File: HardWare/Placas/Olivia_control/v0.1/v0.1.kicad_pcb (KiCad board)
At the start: 2 copper layers, 100 x 100 mm, 47 parts, among them J1 PROG, J10 Motor_B, J11 I2C, J12 DAC, J13 UART2, J15 TRIAC_220VAC, J17 In12V, J2 Input1, J3 Input2, J4 Input3, J5 Input4, J6 LED, J7 Reset, J8 SPI, J9 Motor_A, Q1 BTA16-800B, Q2 BTA16-800B, U1 ESP32-WROOM-32D, U2 MOC3041M, U3 MOC3041M, U4 4N25, U5 AMS1117-3.3, U6 HW-613

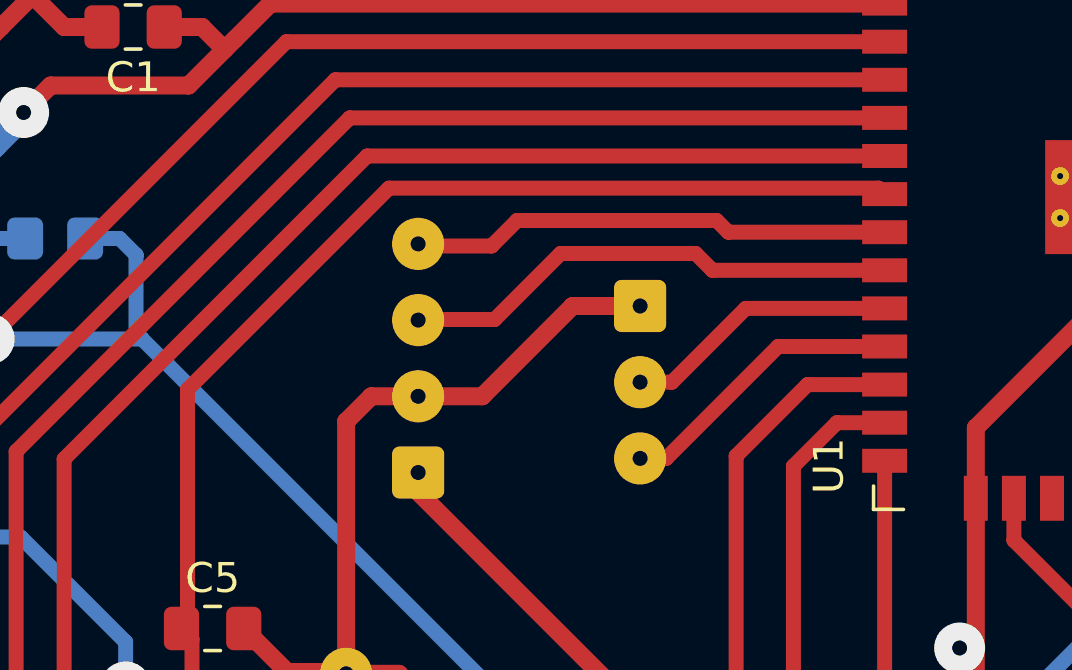
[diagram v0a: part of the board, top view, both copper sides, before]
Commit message: minor fix
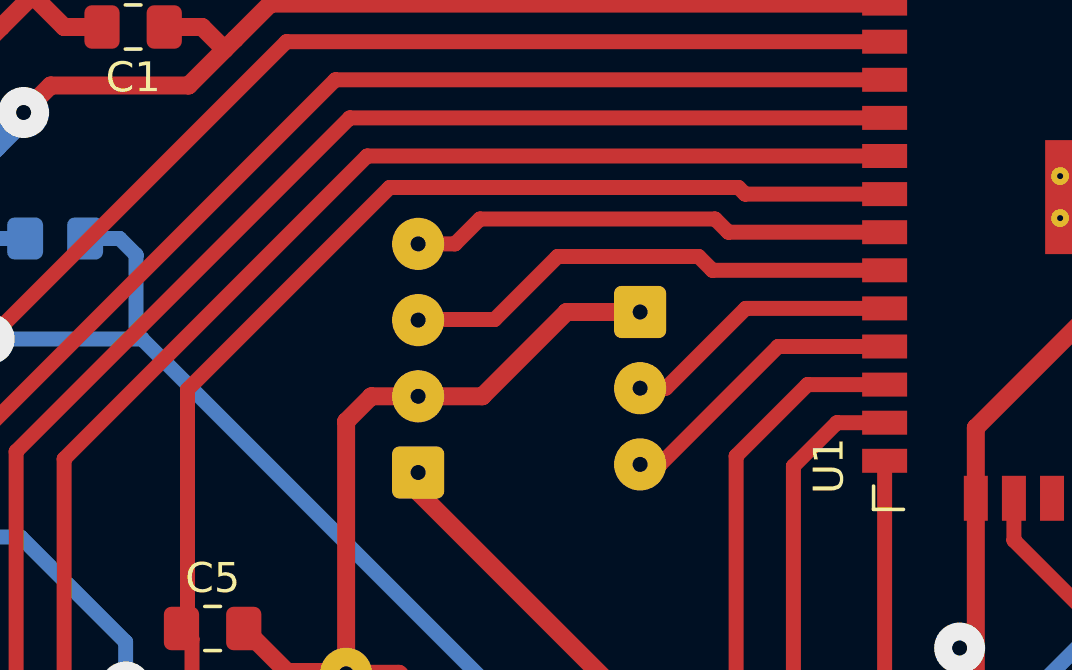
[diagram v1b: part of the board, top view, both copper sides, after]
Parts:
- moved J12 0.20 mm to (129.8, 58.1)
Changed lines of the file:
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@@
 		(allow_soldermask_bridges_in_footprints no)
 		(pcbplotparams
-			(layerselection 0x0000000_fffffffe)
+			(layerselection 0x0000000_7fffffff)
 			(plot_on_all_layers_selection 0x0001000_00000000)
 			(disableapertmacros no)
@@
 			(subtractmaskfromsilk no)
 			(outputformat 4)
-			(mirror yes)
+			(mirror no)
 			(drillshape 2)
 			(scaleselection 1)
@@
 	(footprint "Connector_Molex:Molex_SL_171971-0003_1x03_P2.54mm_Vertical"
 		(layer "B.Cu")
-		(at 129.8 57.9 -90)
+		(at 129.8 58.1 -90)
 		(descr "Molex Stackable Linear Connector, 171971-0003 (compatible alternatives: 171971-0103, 171971-0203), 3 Pins per row (https://www.molex.com/pdm_docs/sd/1719710002_sd.pdf), generated with kicad-footprint-generator")
 		(tags "connector Molex SL vertical")
@@
 	)
 	(segment
-		(start 116.7375 79.5)
-		(end 119.9775 79.5)
+		(start 122.4 60.91)
+		(end 124.54 60.91)
 		(width 0.6)
 		(layer "F.Cu")
@@
 	)
 	(segment
-		(start 122.4 60.91)
-		(end 124.54 60.91)
+		(start 116.7375 79.5)
+		(end 119.9775 79.5)
 		(width 0.6)
 		(layer "F.Cu")
@@
 	)
 	(segment
+		(start 127.35 58.1)
+		(end 129.8 58.1)
+		(width 0.6)
+		(layer "F.Cu")
+		(net 2)
+	)
+	(segment
 		(start 121.39 98.21)
 		(end 119.9875 98.21)
@@
 	)
 	(segment
-		(start 124.54 60.91)
-		(end 127.55 57.9)
-		(width 0.6)
-		(layer "F.Cu")
-		(net 2)
-	)
-	(segment
 		(start 120.0375 88.86)
 		(end 121.86 88.86)
@@
 	)
 	(segment
-		(start 127.55 57.9)
-		(end 129.8 57.9)
-		(width 0.6)
-		(layer "F.Cu")
-		(net 2)
-	)
-	(segment
 		(start 110.55 46.55)
 		(end 145.9 46.55)
@@
 	)
 	(segment
+		(start 124.54 60.91)
+		(end 127.35 58.1)
+		(width 0.6)
+		(layer "F.Cu")
+		(net 2)
+	)
+	(segment
 		(start 134.65 100.95)
 		(end 135.34 100.26)
@@
 	)
 	(segment
-		(start 137.751263 53.971263)
-		(end 137.95 54.17)
+		(start 114.5125 68.65)
+		(end 114.7125 68.45)
+		(width 0.5)
+		(layer "F.Cu")
+		(net 6)
+	)
+	(segment
+		(start 114.8625 69)
+		(end 114.8625 72.54)
 		(width 0.5)
 		(layer "F.Cu")
@@
 	(segment
 		(start 114.7125 60.6875)
-		(end 121.428737 53.971263)
+		(end 121.45 53.95)
 		(width 0.5)
 		(layer "F.Cu")
@@
 	)
 	(segment
-		(start 114.8625 69)
-		(end 114.8625 72.54)
+		(start 121.45 53.95)
+		(end 133.08 53.95)
 		(width 0.5)
 		(layer "F.Cu")
@@
 	)
 	(segment
-		(start 114.7125 68.45)
-		(end 114.7125 60.6875)
+		(start 133.3 54.17)
+		(end 137.95 54.17)
 		(width 0.5)
 		(layer "F.Cu")
@@
 	)
 	(segment
-		(start 114.6625 72.74)
-		(end 119.96 72.74)
+		(start 133.08 53.95)
+		(end 133.3 54.17)
 		(width 0.5)
 		(layer "F.Cu")
@@
 	)
 	(segment
-		(start 114.5125 68.65)
-		(end 114.8625 69)
+		(start 114.6625 72.74)
+		(end 119.96 72.74)
 		(width 0.5)
 		(layer "F.Cu")
@@
 	)
 	(segment
-		(start 114.5125 68.65)
-		(end 114.7125 68.45)
+		(start 114.7125 68.45)
+		(end 114.7125 60.6875)
 		(width 0.5)
 		(layer "F.Cu")
@@
 	)
 	(segment
-		(start 119.96 72.74)
-		(end 120 72.7)
+		(start 114.5125 68.65)
+		(end 114.8625 69)
 		(width 0.5)
 		(layer "F.Cu")
@@
 	)
 	(segment
-		(start 121.428737 53.971263)
-		(end 137.751263 53.971263)
+		(start 119.96 72.74)
+		(end 120 72.7)
 		(width 0.5)
 		(layer "F.Cu")
@@
 	)
 	(segment
-		(start 124.85 55.9)
-		(end 122.47 55.9)
+		(start 124.460365 55)
+		(end 123.630365 55.83)
 		(width 0.5)
 		(layer "F.Cu")
@@
 	)
 	(segment
-		(start 125.7 55.05)
-		(end 124.85 55.9)
+		(start 132.3 55)
+		(end 124.460365 55)
 		(width 0.5)
 		(layer "F.Cu")
@@
 	)
 	(segment
-		(start 132.35 55.05)
-		(end 125.7 55.05)
+		(start 132.74 55.44)
+		(end 132.3 55)
 		(width 0.5)
 		(layer "F.Cu")
@@
 	)
 	(segment
-		(start 122.47 55.9)
+		(start 123.630365 55.83)
 		(end 122.4 55.83)
 		(width 0.5)
@@
 	)
 	(segment
-		(start 132.74 55.44)
-		(end 132.35 55.05)
-		(width 0.5)
-		(layer "F.Cu")
-		(net 28)
-	)
-	(segment
 		(start 137.85 55.44)
 		(end 132.74 55.44)
@@
 	)
 	(segment
-		(start 124.95 58.35)
-		(end 127.15 56.15)
+		(start 132.21 56.71)
+		(end 137.85 56.71)
 		(width 0.5)
 		(layer "F.Cu")
@@
 	)
 	(segment
-		(start 122.4 58.37)
-		(end 122.42 58.35)
+		(start 131.75 56.25)
+		(end 132.21 56.71)
 		(width 0.5)
 		(layer "F.Cu")
@@
 	)
 	(segment
-		(start 131.65 56.15)
-		(end 132.21 56.71)
+		(start 124.95 58.35)
+		(end 127.05 56.25)
 		(width 0.5)
 		(layer "F.Cu")
@@
 	)
 	(segment
-		(start 132.21 56.71)
-		(end 137.85 56.71)
+		(start 122.42 58.35)
+		(end 124.95 58.35)
 		(width 0.5)
 		(layer "F.Cu")
@@
 	)
 	(segment
-		(start 122.42 58.35)
-		(end 124.95 58.35)
+		(start 127.05 56.25)
+		(end 131.75 56.25)
 		(width 0.5)
 		(layer "F.Cu")
@@
 	)
 	(segment
-		(start 127.15 56.15)
-		(end 131.65 56.15)
+		(start 122.4 58.37)
+		(end 122.42 58.35)
 		(width 0.5)
 		(layer "F.Cu")
@@
 	(segment
 		(start 133.32 57.98)
-		(end 130.86 60.44)
+		(end 130.66 60.64)
 		(width 0.5)
 		(layer "F.Cu")
@@
 	)
 	(segment
-		(start 130.86 60.44)
-		(end 129.8 60.44)
+		(start 137.85 57.98)
+		(end 133.32 57.98)
 		(width 0.5)
 		(layer "F.Cu")
@@
 	)
 	(segment
-		(start 137.85 57.98)
-		(end 133.32 57.98)
+		(start 130.66 60.64)
+		(end 129.8 60.64)
 		(width 0.5)
 		(layer "F.Cu")
@@
 	)
 	(segment
-		(start 137.85 59.25)
-		(end 134.4 59.25)
+		(start 134.4 59.25)
+		(end 130.47 63.18)
 		(width 0.5)
 		(layer "F.Cu")
@@
 	)
 	(segment
-		(start 134.4 59.25)
-		(end 130.67 62.98)
+		(start 130.47 63.18)
+		(end 129.8 63.18)
 		(width 0.5)
 		(layer "F.Cu")
@@
 	)
 	(segment
-		(start 130.67 62.98)
-		(end 129.8 62.98)
+		(start 137.85 59.25)
+		(end 134.4 59.25)
 		(width 0.5)
 		(layer "F.Cu")
